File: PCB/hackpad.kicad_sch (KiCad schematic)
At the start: 21 parts, among them SW1 SW_Push, SW10 RotaryEncoder_Switch, SW11 SW_Push, SW12 SW_Push, SW13 SW_Push, SW14 SW_Push, SW15 SW_Push, SW16 SW_Push, SW17 SW_Push, SW2 SW_Push, SW3 SW_Push, SW4 SW_Push, SW5 SW_Push, SW6 SW_Push, SW7 SW_Push, SW8 SW_Push, SW9 SW_Push, U1 MOUDLE-SEEEDUINO-XIAO, U2 MCP23017x-x-SO

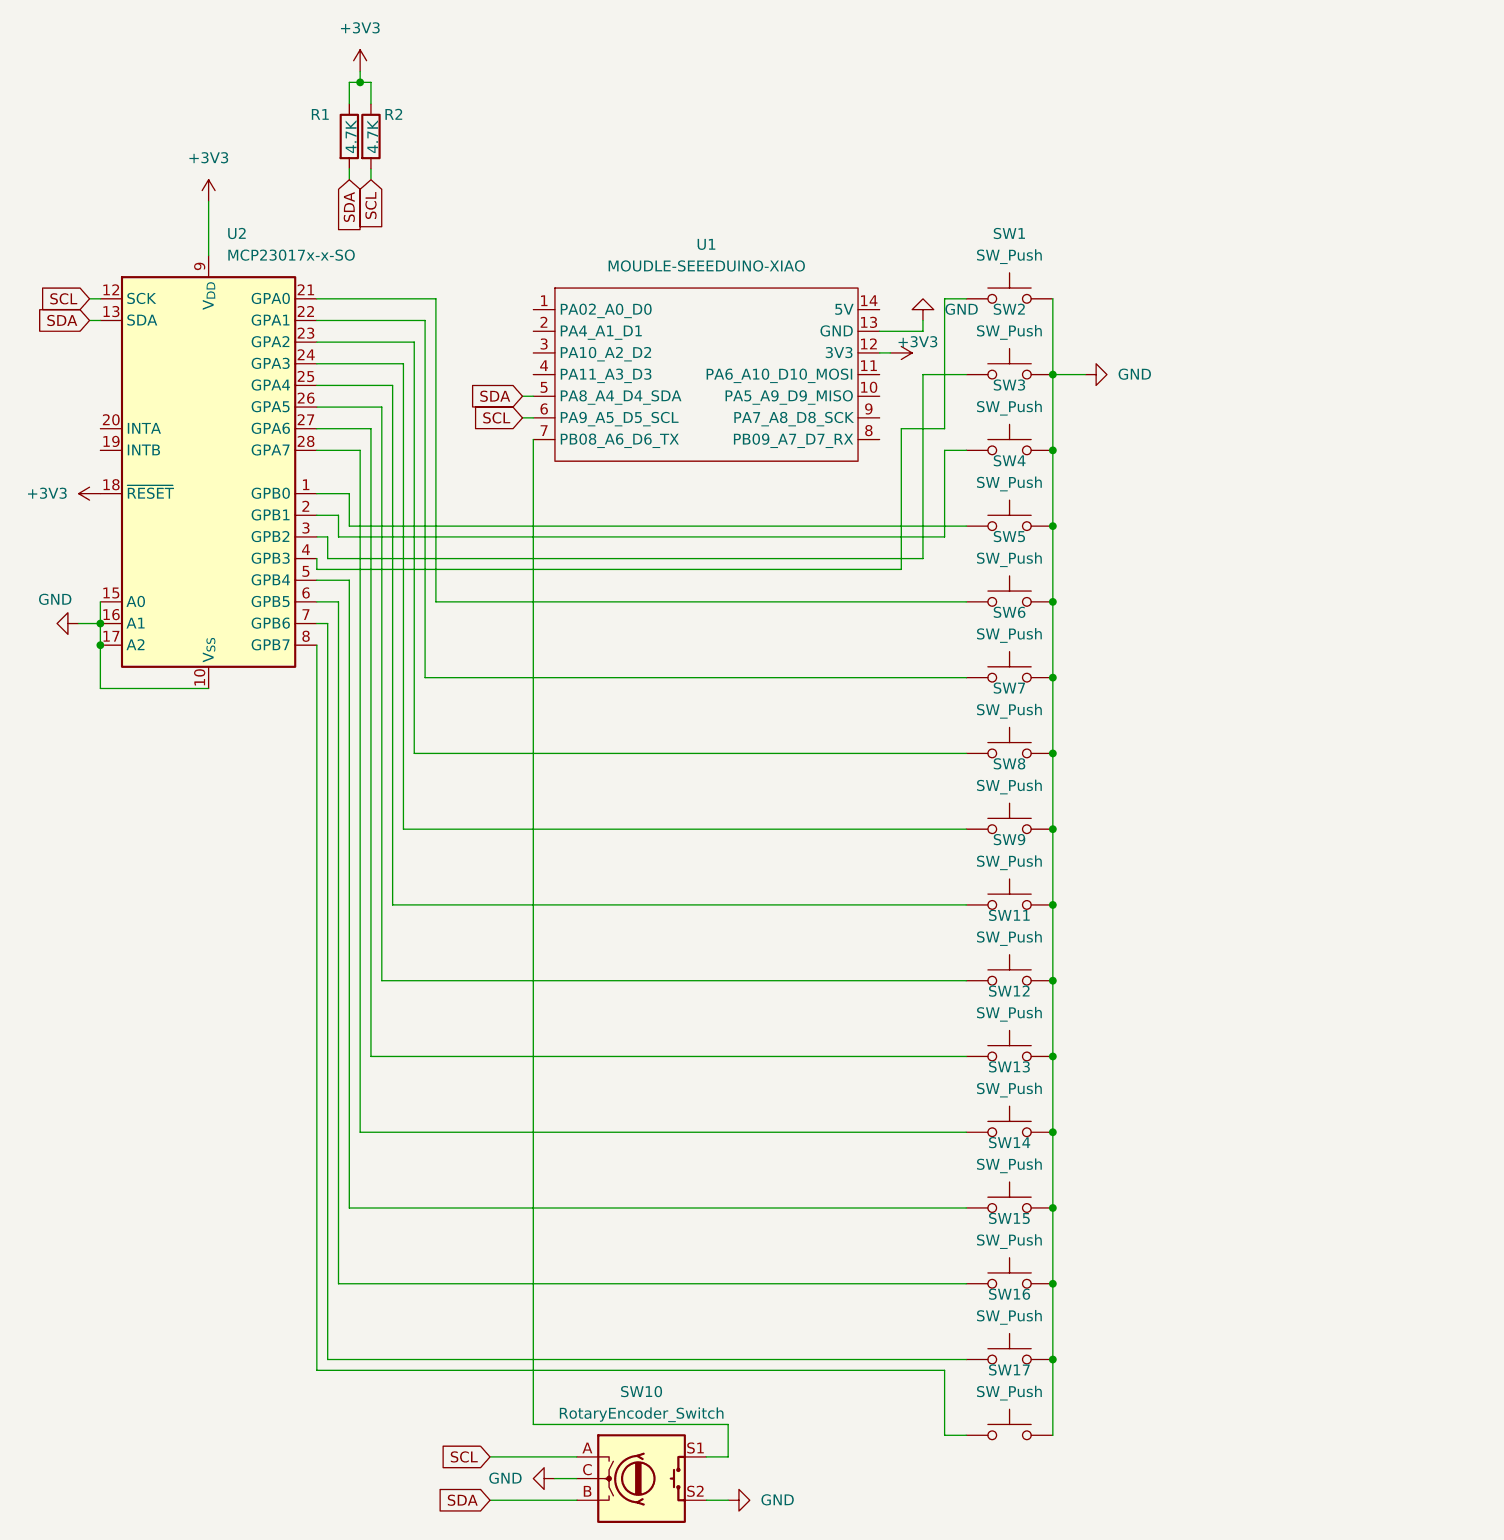
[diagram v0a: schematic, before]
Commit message: Diode matrix
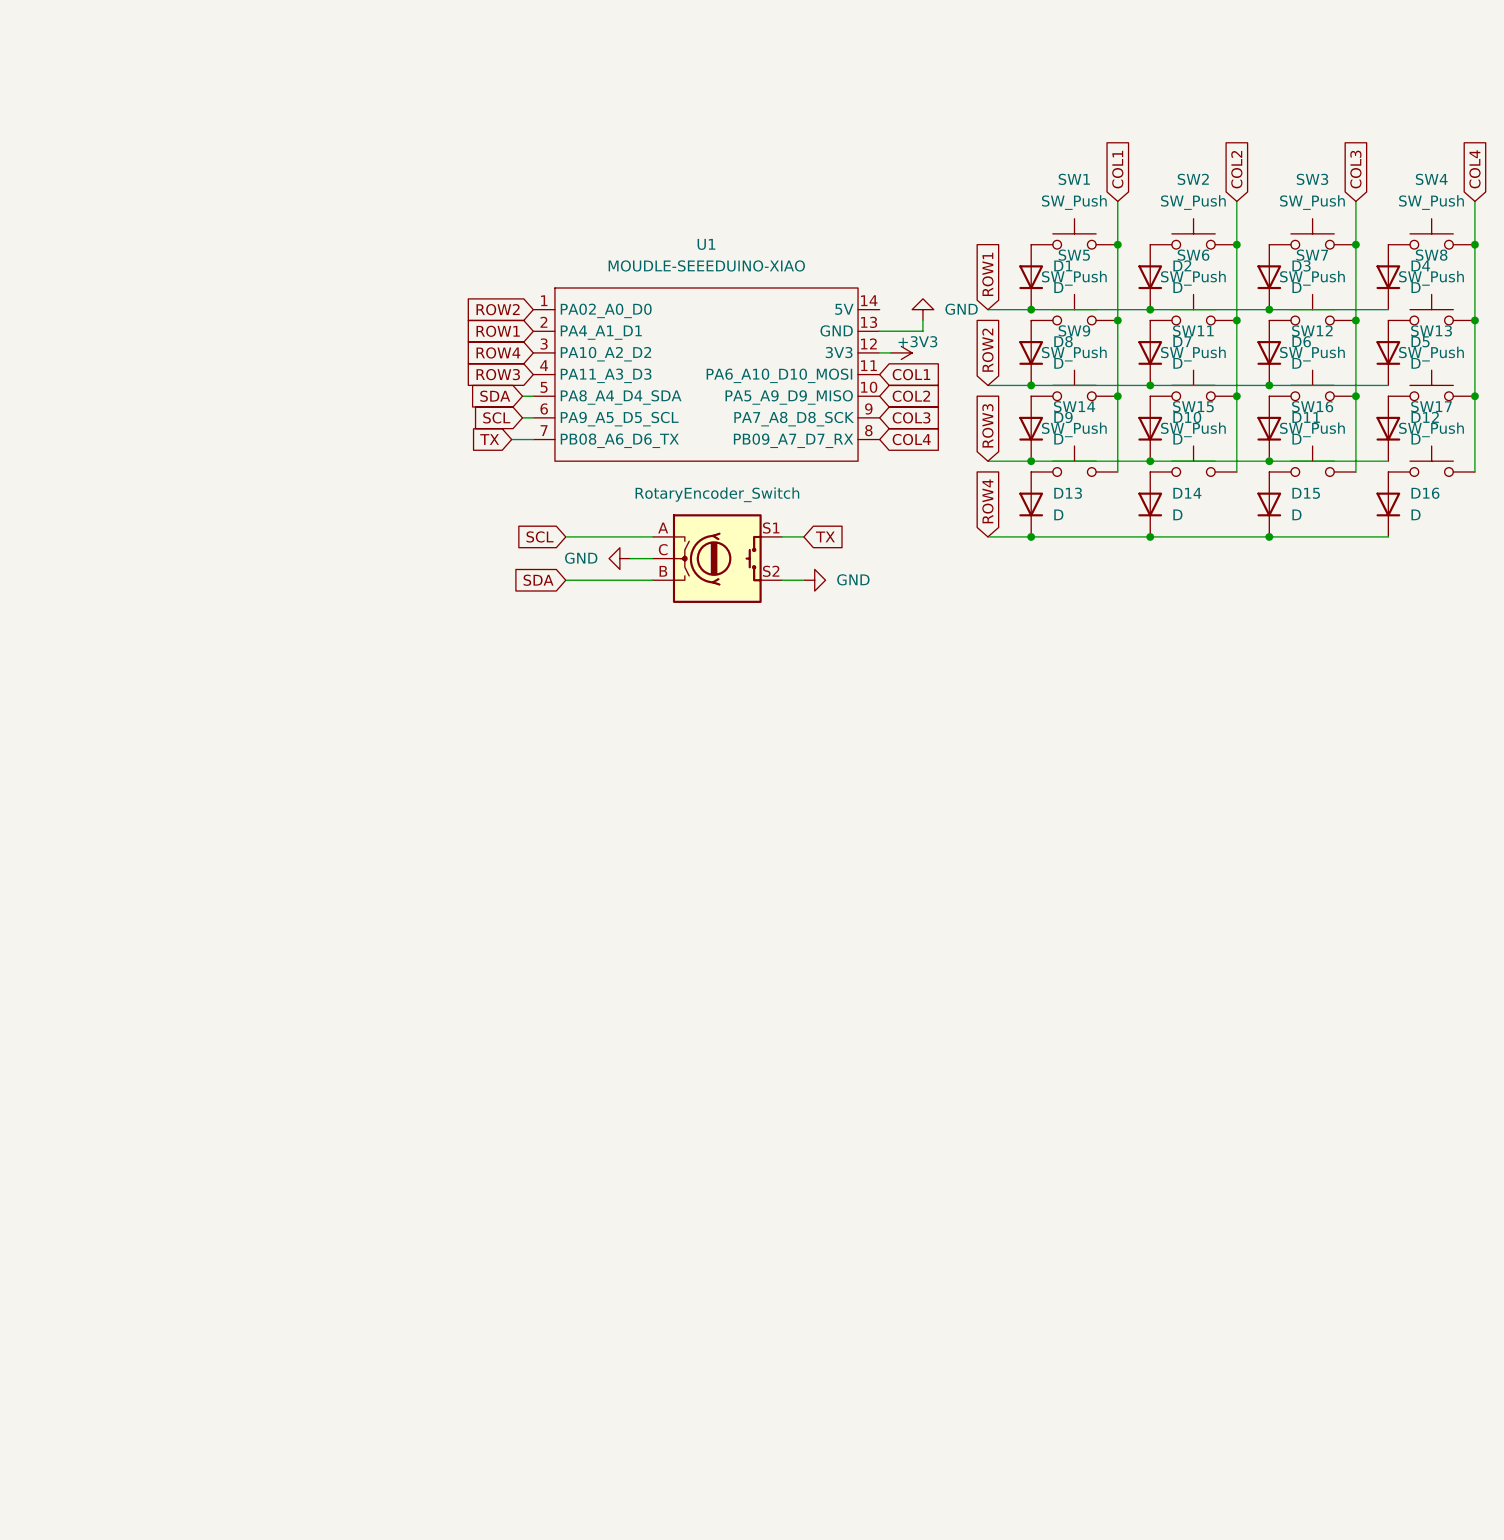
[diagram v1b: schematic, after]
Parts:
- removed R1, R2: 4.7K, Resistor_THT:R_Axial_DIN0204_L3.6mm_D1.6mm_P7.62mm_Horizontal, symbol Device:R
- removed U2: MCP23017x-x-SO, Package_SO:SOIC-28W_7.5x17.9mm_P1.27mm, symbol Interface_Expansion:MCP23017x-x-SO
- added D1, D10, D11, D12, D13, D14, D15, D16, D2, D3, D4, D5, D6, D7, D8, D9: D, Diode_THT:D_DO-35_SOD27_P7.62mm_Horizontal, symbol Device:D
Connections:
- net GND: no longer SW1.2, SW11.2, SW12.2, SW13.2, SW14.2, SW15.2, SW16.2, SW17.2, SW2.2, SW3.2, SW4.2, SW5.2, SW6.2, SW7.2, SW8.2, SW9.2
- net ROW2: now reaches U1.1 (PA02_A0_D0)
- net ROW2: now also D5.1 (K), D6.1 (K), D7.1 (K), D8.1 (K)
- net COL2: now reaches U1.10 (PA5_A9_D9_MISO)
- net COL2: now also SW11.2, SW15.2, SW2.2, SW6.2
- net COL1: now reaches U1.11 (PA6_A10_D10_MOSI)
- net COL1: now also SW1.2, SW14.2, SW5.2, SW9.2
- net ROW1: now reaches U1.2 (PA4_A1_D1)
- net ROW1: now also D1.1 (K), D2.1 (K), D3.1 (K), D4.1 (K)
- net ROW4: now reaches U1.3 (PA10_A2_D2)
- net ROW4: now also D13.1 (K), D14.1 (K), D15.1 (K), D16.1 (K)
- net ROW3: now reaches U1.4 (PA11_A3_D3)
- net ROW3: now also D10.1 (K), D11.1 (K), D12.1 (K), D9.1 (K)
- net TX: now reaches SW10.S1, U1.7 (PB08_A6_D6_TX)
- net COL4: now reaches U1.8 (PB09_A7_D7_RX)
- net COL4: now also SW13.2, SW17.2, SW4.2, SW8.2
- net COL3: now reaches U1.9 (PA7_A8_D8_SCK)
- net COL3: now also SW12.2, SW16.2, SW3.2, SW7.2
- net at SW1.1: now also D1.2 (A)
- net at SW12.1: now also D11.2 (A)
- net at SW2.1: now also D2.2 (A)
- net at SW13.1: now also D12.2 (A)
- net at SW3.1: now also D3.2 (A)
- net at SW8.1: now also D5.2 (A)
- net at SW16.1: now also D15.2 (A)
- net at SW7.1: now also D6.2 (A)
- net at SW6.1: now also D7.2 (A)
- net at SW9.1: now also D9.2 (A)
- net at SW4.1: now also D4.2 (A)
- net at SW5.1: now also D8.2 (A)
- net at SW11.1: now also D10.2 (A)
- net at SW14.1: now also D13.2 (A)
- net at SW15.1: now also D14.2 (A)
- net at SW17.1: now also D16.2 (A)
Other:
- moved on the sheet: SW1, SW11, SW12, SW13, SW14, SW15, SW16, SW17, SW2, SW3, SW4, SW5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
